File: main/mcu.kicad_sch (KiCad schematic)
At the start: 16 parts, among them J501 Conn_ARM_JTAG_SWD_20, J502 Debug, SW501 B3SL-1022P, U501 STM32L476RGTx, Y501 8MHz

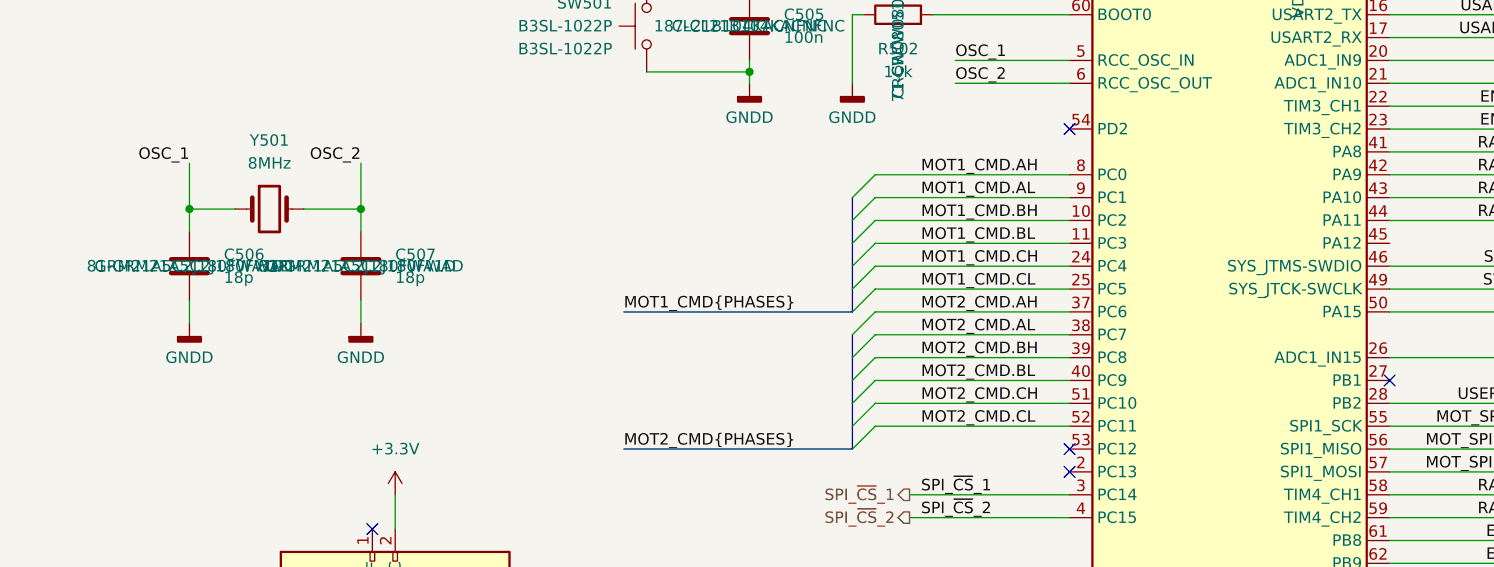
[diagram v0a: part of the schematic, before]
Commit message: Revised with BOM ordered
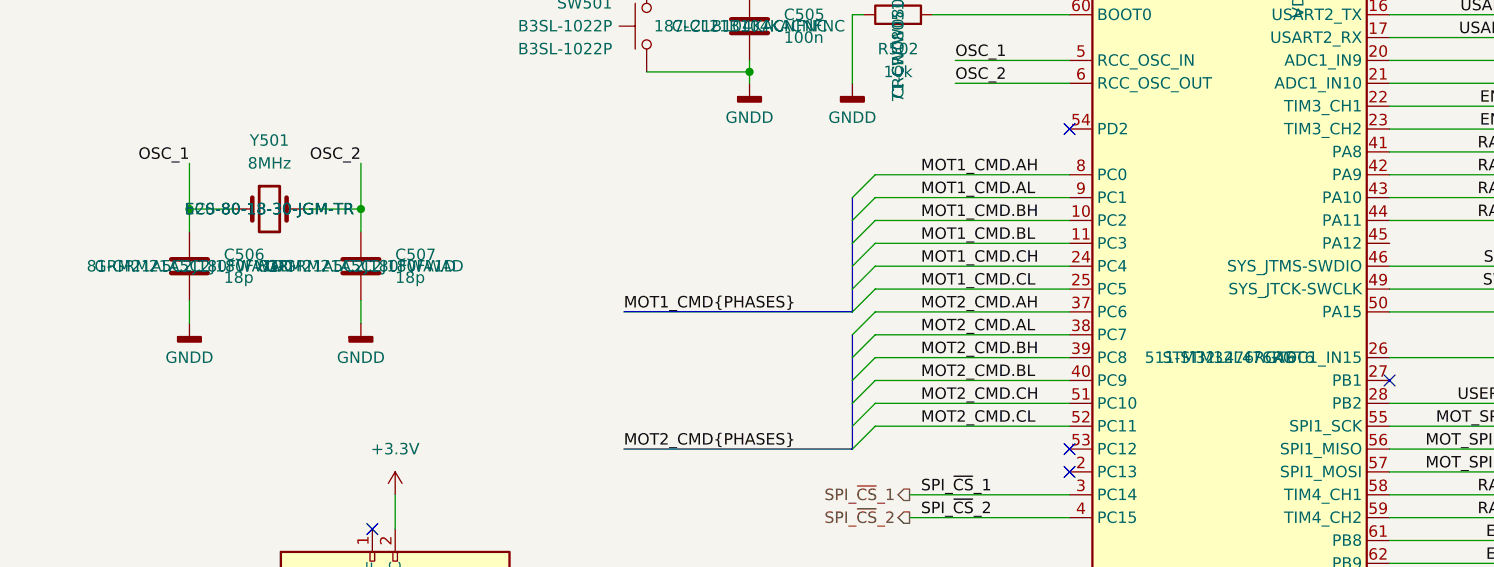
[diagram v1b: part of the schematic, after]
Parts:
- C501, C502, C503, C504, C505: Mouser SKU 187-CL21B104KACNFNC -> 187-CL21B104KACNFNC
- C506, C507: Mouser SKU 81-GRM21A5C2J180FWAD -> 81-GRM21A5C2J180FWAD
- U501: MPN (none) -> STM32L476RGT6; Mouser SKU (none) -> 511-STM32L476RGT6
- Y501: MPN (none) -> ECS-80-18-30-JGM-TR; Mouser SKU (none) -> 520-80-18-30-JGM-TR
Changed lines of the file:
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@@
 			)
 		)
-		(property "Mouser SKU" " 187-CL21B104KACNFNC "
+		(property "Mouser SKU" "187-CL21B104KACNFNC "
 			(at 63.5 29.21 0)
 			(effects
@@
 			)
 		)
-		(property "Mouser SKU" " 81-GRM21A5C2J180FWAD "
+		(property "Mouser SKU" "81-GRM21A5C2J180FWAD "
 			(at 46.99 76.2 0)
 			(effects
@@
 			)
 		)
-		(property "Mouser SKU" " 81-GRM21A5C2J180FWAD "
+		(property "Mouser SKU" "81-GRM21A5C2J180FWAD "
 			(at 27.94 76.2 0)
 			(effects
@@
 			)
 		)
-		(property "Mouser SKU" " 187-CL21B104KACNFNC "
+		(property "Mouser SKU" "187-CL21B104KACNFNC "
 			(at 35.56 29.21 0)
 			(effects
@@
 			)
 		)
+		(property "MPN" "ECS-80-18-30-JGM-TR "
+			(at 36.83 69.85 0)
+			(effects
+				(font
+					(size 1.27 1.27)
+				)
+			)
+		)
+		(property "Name" ""
+			(at 36.83 69.85 0)
+			(effects
+				(font
+					(size 1.27 1.27)
+				)
+			)
+		)
+		(property "Mouser SKU" " 520-80-18-30-JGM-TR "
+			(at 36.83 69.85 0)
+			(effects
+				(font
+					(size 1.27 1.27)
+				)
+			)
+		)
 		(pin "1"
 		)
@@
 			)
 		)
-		(property "Mouser SKU" " 187-CL21B104KACNFNC "
+		(property "Mouser SKU" "187-CL21B104KACNFNC "
 			(at 90.17 49.53 0)
 			(effects
@@
 			)
 		)
-		(property "MPN" ""
+		(property "MPN" "STM32L476RGT6"
 			(at 143.51 86.36 0)
 			(effects
@@
 			)
 		)
+		(property "Mouser SKU" " 511-STM32L476RGT6 "
+			(at 143.51 86.36 0)
+			(effects
+				(font
+					(size 1.27 1.27)
+				)
+			)
+		)
 		(pin "30"
 		)
@@
 			)
 		)
-		(property "Mouser SKU" " 187-CL21B104KACNFNC "
+		(property "Mouser SKU" "187-CL21B104KACNFNC "
 			(at 49.53 29.21 0)
 			(effects
@@
 			)
 		)
-		(property "Mouser SKU" " 187-CL21B104KACNFNC "
+		(property "Mouser SKU" "187-CL21B104KACNFNC "
 			(at 21.59 29.21 0)
 			(effects
